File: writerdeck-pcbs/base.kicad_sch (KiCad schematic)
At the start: 4 parts, among them J2 12401826E412A

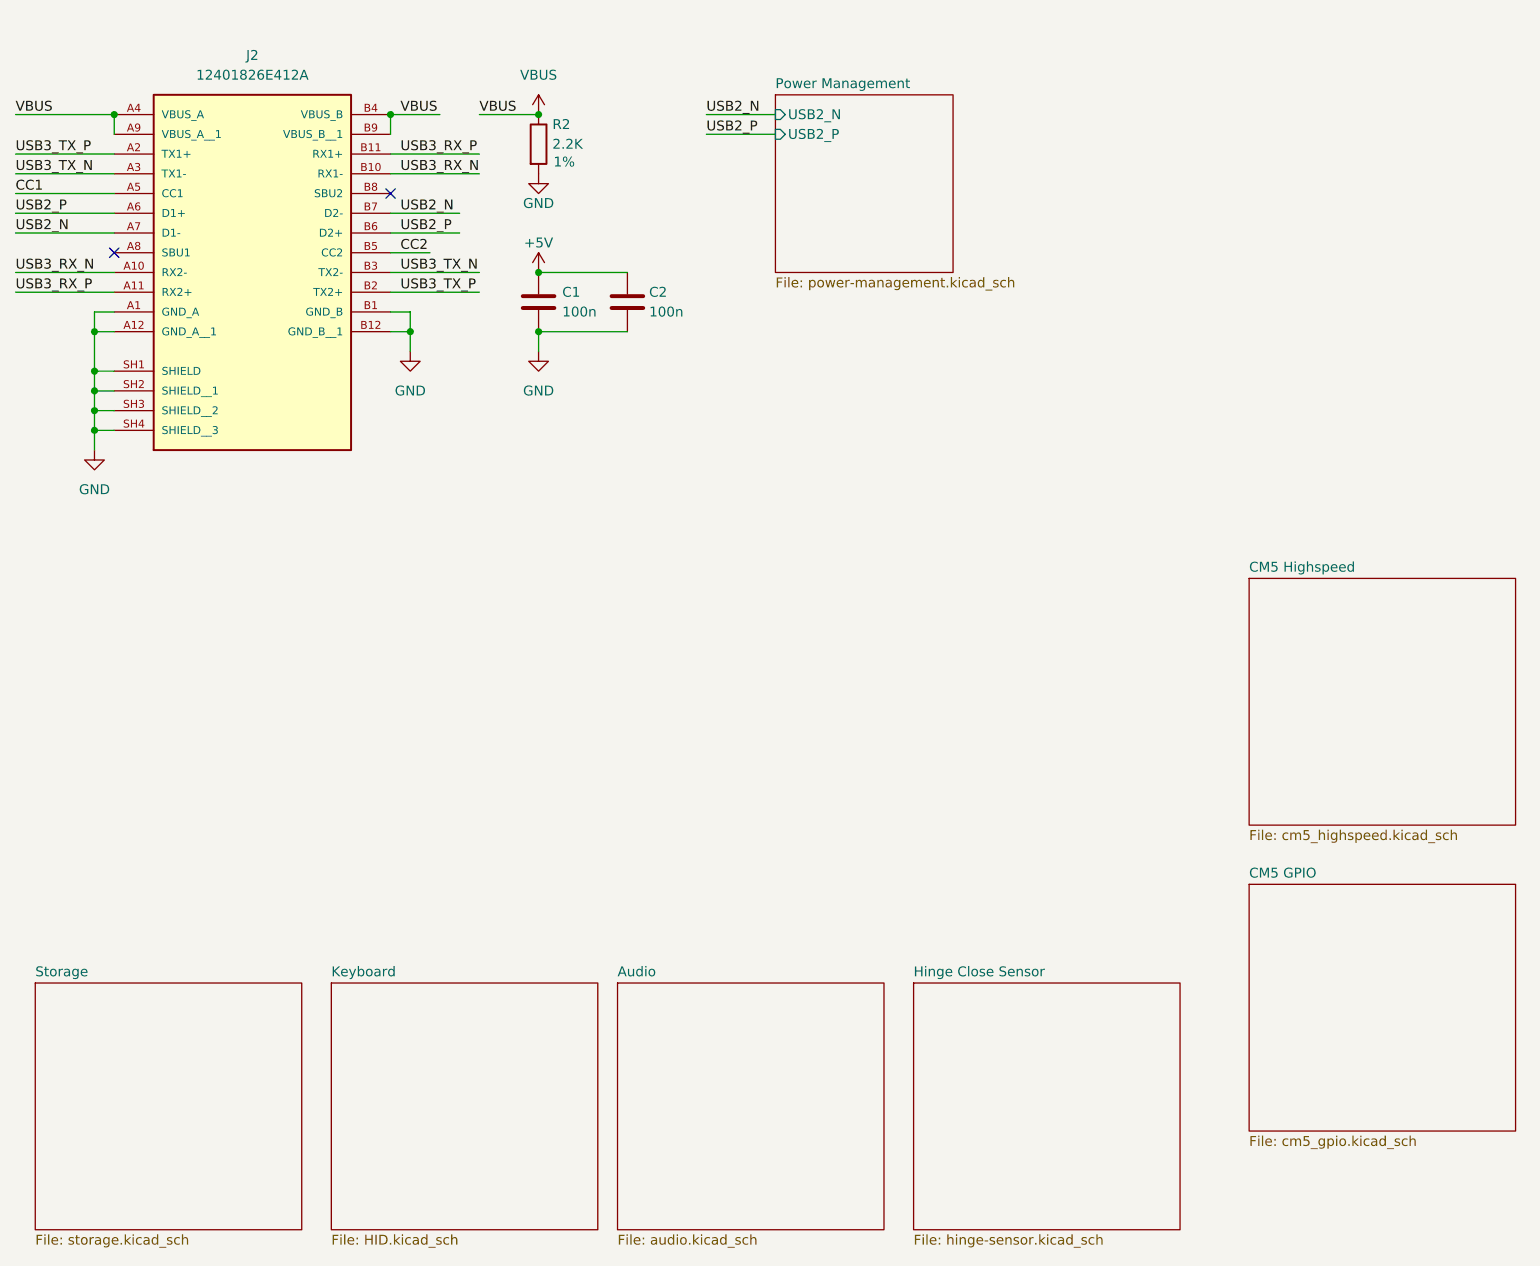
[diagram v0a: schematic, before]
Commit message: power management done
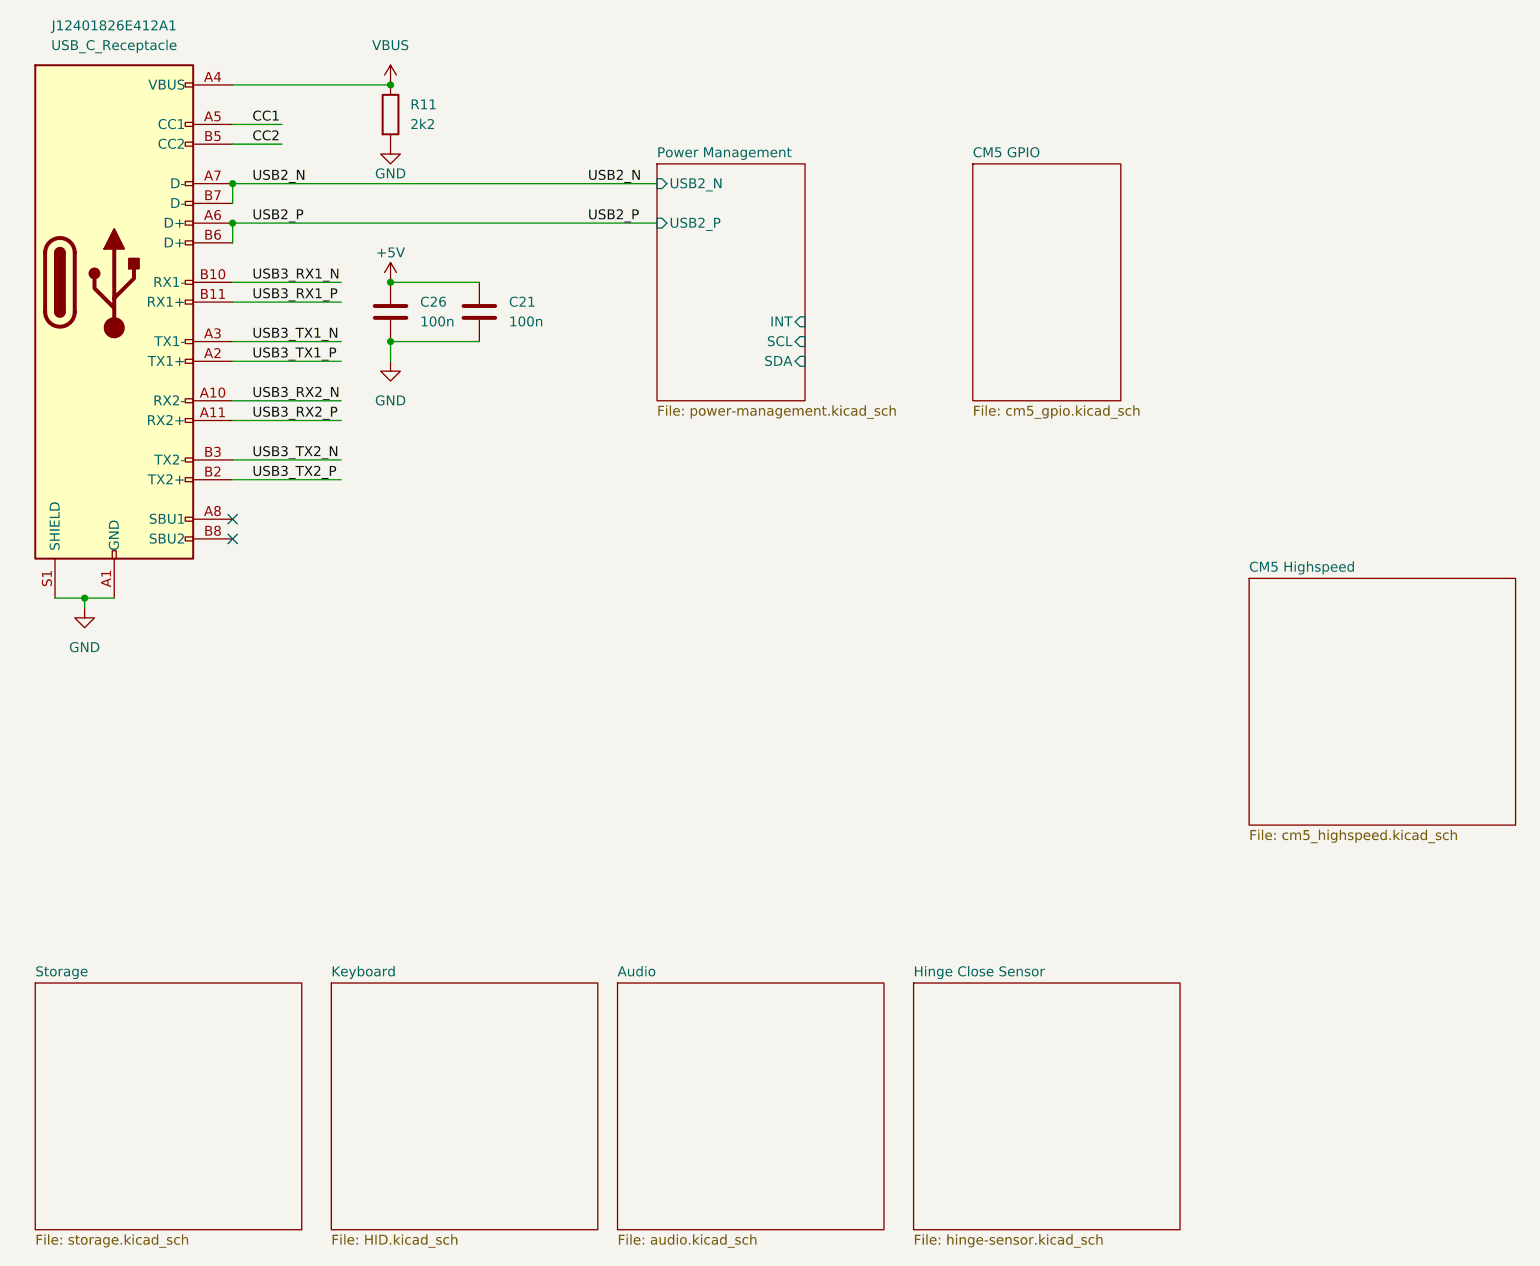
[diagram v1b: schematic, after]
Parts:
- removed C1, C2: 100n, symbol Device:C
- removed J2: 12401826E412A, ZF_common:12401826E412A, symbol ZF_common:12401826E412A
- removed R2: 2.2K, symbol Device:R
- added C21, C26: 100n, Capacitor_SMD:C_0603_1608Metric, symbol ZF_common:100n 5% 0603 Capacitor
- added J12401826E412A1: USB_C_Receptacle, ZF_common:12401826E412A, symbol Connector:USB_C_Receptacle
- added R11: 2k2, Resistor_SMD:R_0603_1608Metric, symbol ZF_common:2k2 1% 0603 Resistor
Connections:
- net +5V: now also C21.1, C26.1
- net CC1: now also J12401826E412A1.A5 (CC1)
- net CC2: now also J12401826E412A1.B5 (CC2)
- net GND: now also C21.2, C26.2, J12401826E412A1.A1 (GND), J12401826E412A1.A12 (GND), J12401826E412A1.B1 (GND), J12401826E412A1.B12 (GND), J12401826E412A1.S1 (SHIELD), R11.2
- net USB2_N: now also J12401826E412A1.A7 (D-), J12401826E412A1.B7 (D-)
- net USB2_P: now also J12401826E412A1.A6 (D+), J12401826E412A1.B6 (D+)
- net VBUS: now also J12401826E412A1.A4 (VBUS), J12401826E412A1.A9 (VBUS), J12401826E412A1.B4 (VBUS), J12401826E412A1.B9 (VBUS), R11.1
- new net USB3_RX1_N: J12401826E412A1.B10 (RX1-)
- new net USB3_RX1_P: J12401826E412A1.B11 (RX1+)
- new net USB3_RX2_N: J12401826E412A1.A10 (RX2-)
- new net USB3_RX2_P: J12401826E412A1.A11 (RX2+)
- new net USB3_TX1_N: J12401826E412A1.A3 (TX1-)
- new net USB3_TX1_P: J12401826E412A1.A2 (TX1+)
- new net USB3_TX2_N: J12401826E412A1.B3 (TX2-)
- new net USB3_TX2_P: J12401826E412A1.B2 (TX2+)
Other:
- sheet Power Management ports: added INT, SCL, SDA; removed none
